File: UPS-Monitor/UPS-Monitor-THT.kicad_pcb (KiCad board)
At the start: 2 copper layers, 46 x 78 mm, 18 parts, among them U1 Xiao ESP32C3, U2 INA260/INA228, U3 Pololu D24V7F3

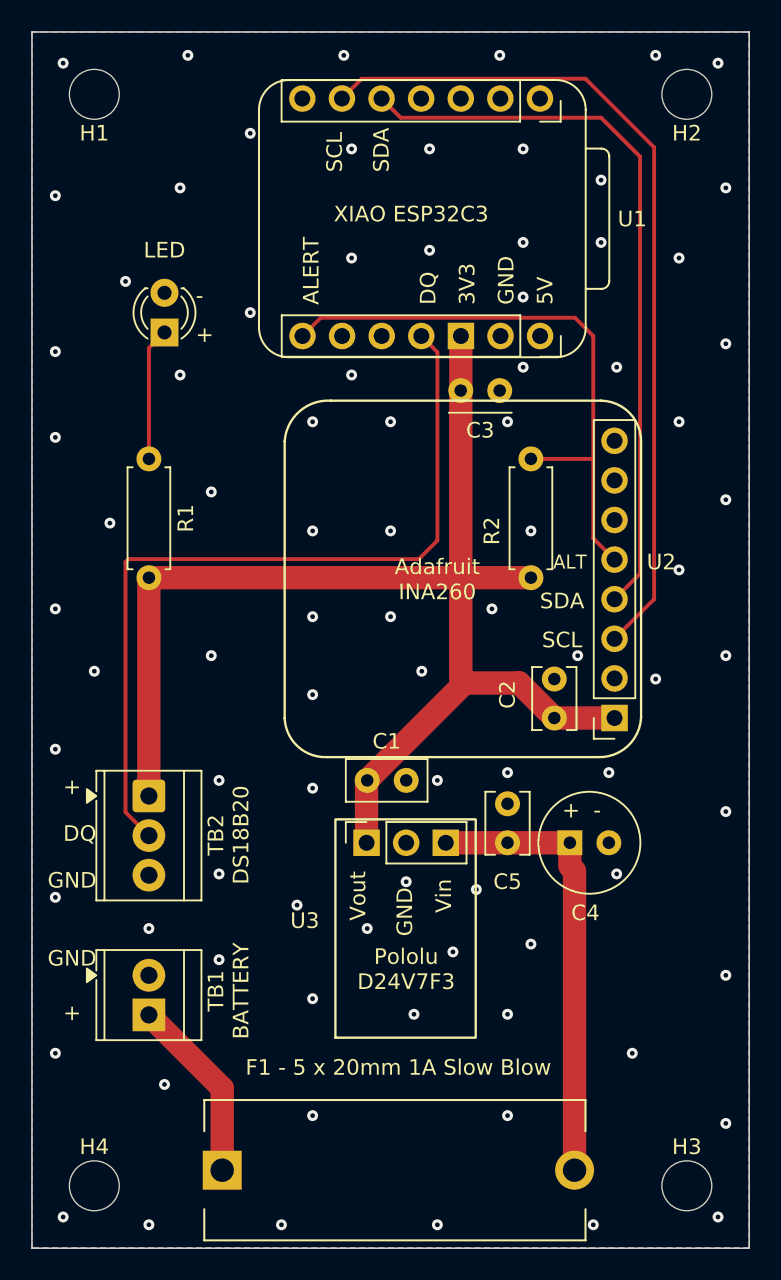
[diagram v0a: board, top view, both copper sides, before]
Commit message: Add files via upload
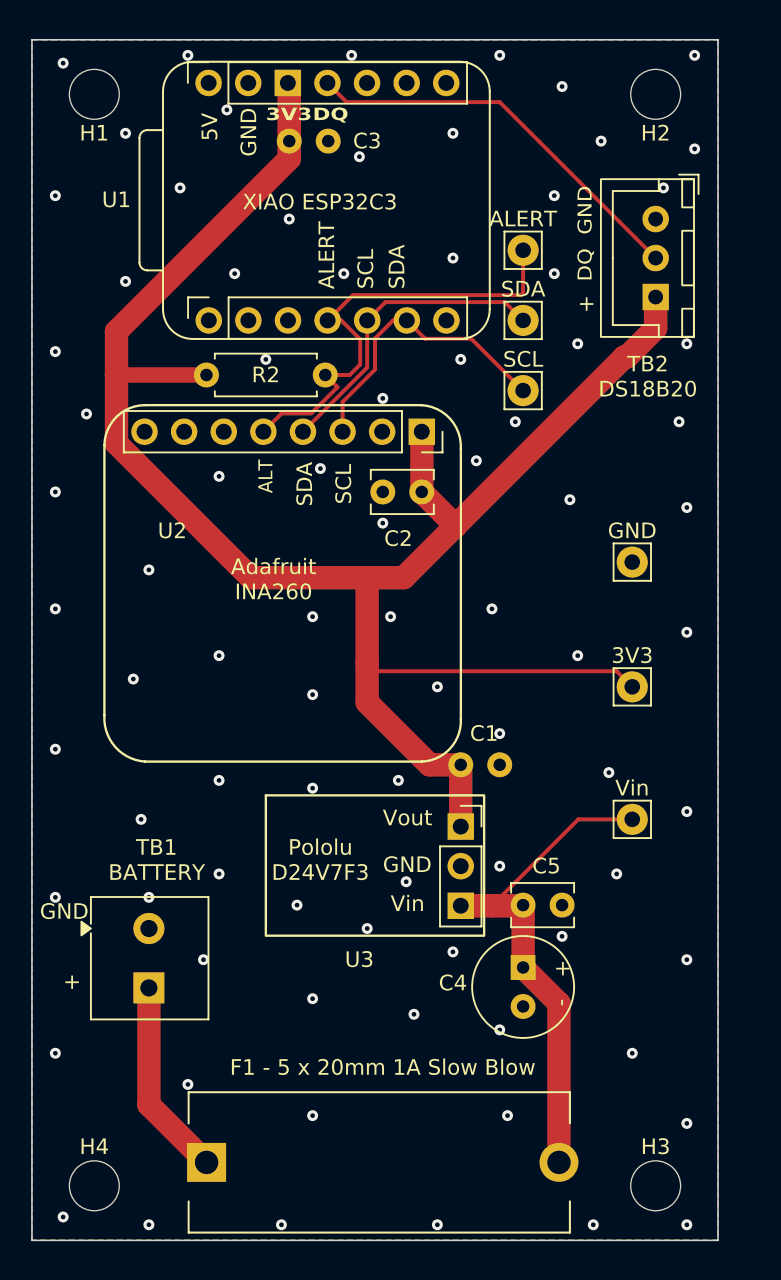
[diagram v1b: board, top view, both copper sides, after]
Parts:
- removed LED: Green 3mm, LED_THT:LED_D3.0mm
- removed R1: 1k 1/4W, Resistor_THT:R_Axial_DIN0207_L6.3mm_D2.5mm_P7.62mm_Horizontal
- added 3V3: TestPoint_THTPad_2.0x2.0mm_Drill1.0mm, TestPoint:TestPoint_THTPad_2.0x2.0mm_Drill1.0mm, F.Cu at (38.5, 47.0)
- added ALERT: TestPoint_THTPad_2.0x2.0mm_Drill1.0mm, TestPoint:TestPoint_THTPad_2.0x2.0mm_Drill1.0mm, F.Cu at (31.5, 19.0)
- added GND: TestPoint_THTPad_2.0x2.0mm_Drill1.0mm, TestPoint:TestPoint_THTPad_2.0x2.0mm_Drill1.0mm, F.Cu at (38.5, 39.0)
- added SCL: TestPoint_THTPad_2.0x2.0mm_Drill1.0mm, TestPoint:TestPoint_THTPad_2.0x2.0mm_Drill1.0mm, F.Cu at (31.5, 28.0)
- added SDA: TestPoint_THTPad_2.0x2.0mm_Drill1.0mm, TestPoint:TestPoint_THTPad_2.0x2.0mm_Drill1.0mm, F.Cu at (31.5, 23.5)
- added Vin: TestPoint_THTPad_2.0x2.0mm_Drill1.0mm, TestPoint:TestPoint_THTPad_2.0x2.0mm_Drill1.0mm, F.Cu at (38.5, 55.5)
- TB1: value TerminalBlock_TE_282834-2_1x02_P2.54mm_Horizontal -> TerminalBlock_Phoenix_MKDS-1-2-3.81_1x02_P3.81mm_Horizontal; footprint TerminalBlock_TE-Connectivity:TerminalBlock_TE_282834-2_1x02_P2.54mm_Horizontal -> TerminalBlock_Phoenix:TerminalBlock_Phoenix_MKDS-1-2-3.81_1x02_P3.81mm_Horizontal
- TB2: value TerminalBlock_TE_282834-3_1x03_P2.54mm_Horizontal -> JST_XH_B3B-XH-A_1x03_P2.50mm_Vertical; footprint TerminalBlock_TE-Connectivity:TerminalBlock_TE_282834-3_1x03_P2.54mm_Horizontal -> Connector_JST:JST_XH_B3B-XH-A_1x03_P2.50mm_Vertical
- moved TB2 49.2 mm to (40.0, 17.0)
- moved U2 22.1 mm to (25.0, 30.6), turned to -90 degrees
- moved C3 19.4 mm to (19.0, 12.0)
- moved U1 17.0 mm to (26.6, 23.5), turned to 180 degrees
- moved C2 16.3 mm to (22.5, 34.5), turned to 0 degrees
- moved R2 14.2 mm to (18.8, 27.0), turned to 180 degrees
- moved C4 8.54 mm to (31.5, 65.0), turned to -90 degrees
- moved C5 7.38 mm to (34.0, 61.0), turned to 180 degrees
- moved U3 6.13 mm to (27.5, 56.0), turned to 0 degrees
- moved C1 6.08 mm to (27.5, 52.0)
- moved TB1 3.00 mm to (7.50, 62.5)
- moved H2 2.00 mm to (40.0, 9.00)
- moved H3 2.00 mm to (40.0, 79.0)
- moved F1 1.12 mm to (22.5, 77.5)
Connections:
- R2 pad 1: GPIO20_ALERT -> GPIO3_ALERT
- TB2 pad 1: +3V3 -> GND
- TB2 pad 3: GND -> +3V3
- U1 pad GPIO20: GPIO20_ALERT -> (no net)
- U2 pad 5: GPIO20_ALERT -> GPIO3_ALERT
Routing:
- net +3V3: track 84.2 -> 124.3 mm
- net GPIO20_ALERT: track 38.5 -> 0.00 mm
- net SCL: track 54.9 -> 18.7 mm
- net GPIO3_ALERT: track 0.00 -> 29.8 mm
- net SDA: track 47.2 -> 19.8 mm
- net GPIO10_DQ: track 52.3 -> 25.7 mm
- net LED_R1: track 8.64 -> 0.00 mm
- net VIN: track 28.7 -> 32.2 mm
- net BATT_RAW: track 11.9 -> 12.7 mm
- net GND: vias 85 -> 84
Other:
- board size 46 x 78 mm -> 44 x 77 mm
- board text added: "Board Size: 44mm x 77mm 1 3/4{dblquote} x 3{dblquote}"
- board text added: "UPS-Monitor-THT.kicad_pcb Rev 1 June 3, 2026 OSH PARK - Fabricator"
- board text removed: "Board Size: 46mm x 78mm 1 13/16{dblquote} x 3 1/16{dblquote}"
- board text removed: "R1 - 1K OHM 5% 1/4W AXIAL"
- board text removed: "{dblquote}UPS-Monitor-THT.kicad_pcb{dblquote} Rev 0 May 14, 2026 OSH PARK - Fabricator"
